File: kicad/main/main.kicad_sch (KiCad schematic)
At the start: 17 parts, among them J2 Conn_01x02, J3 Conn_01x07_Pin, J4 Conn_01x04_Pin, P1 USB_C_Plug_USB2.0, SW1 MK-12C03-G015, SW3 SW_Push, SW4 SW_Push, U1 HUSB237, U2 ZX-PH2.0-WT4P

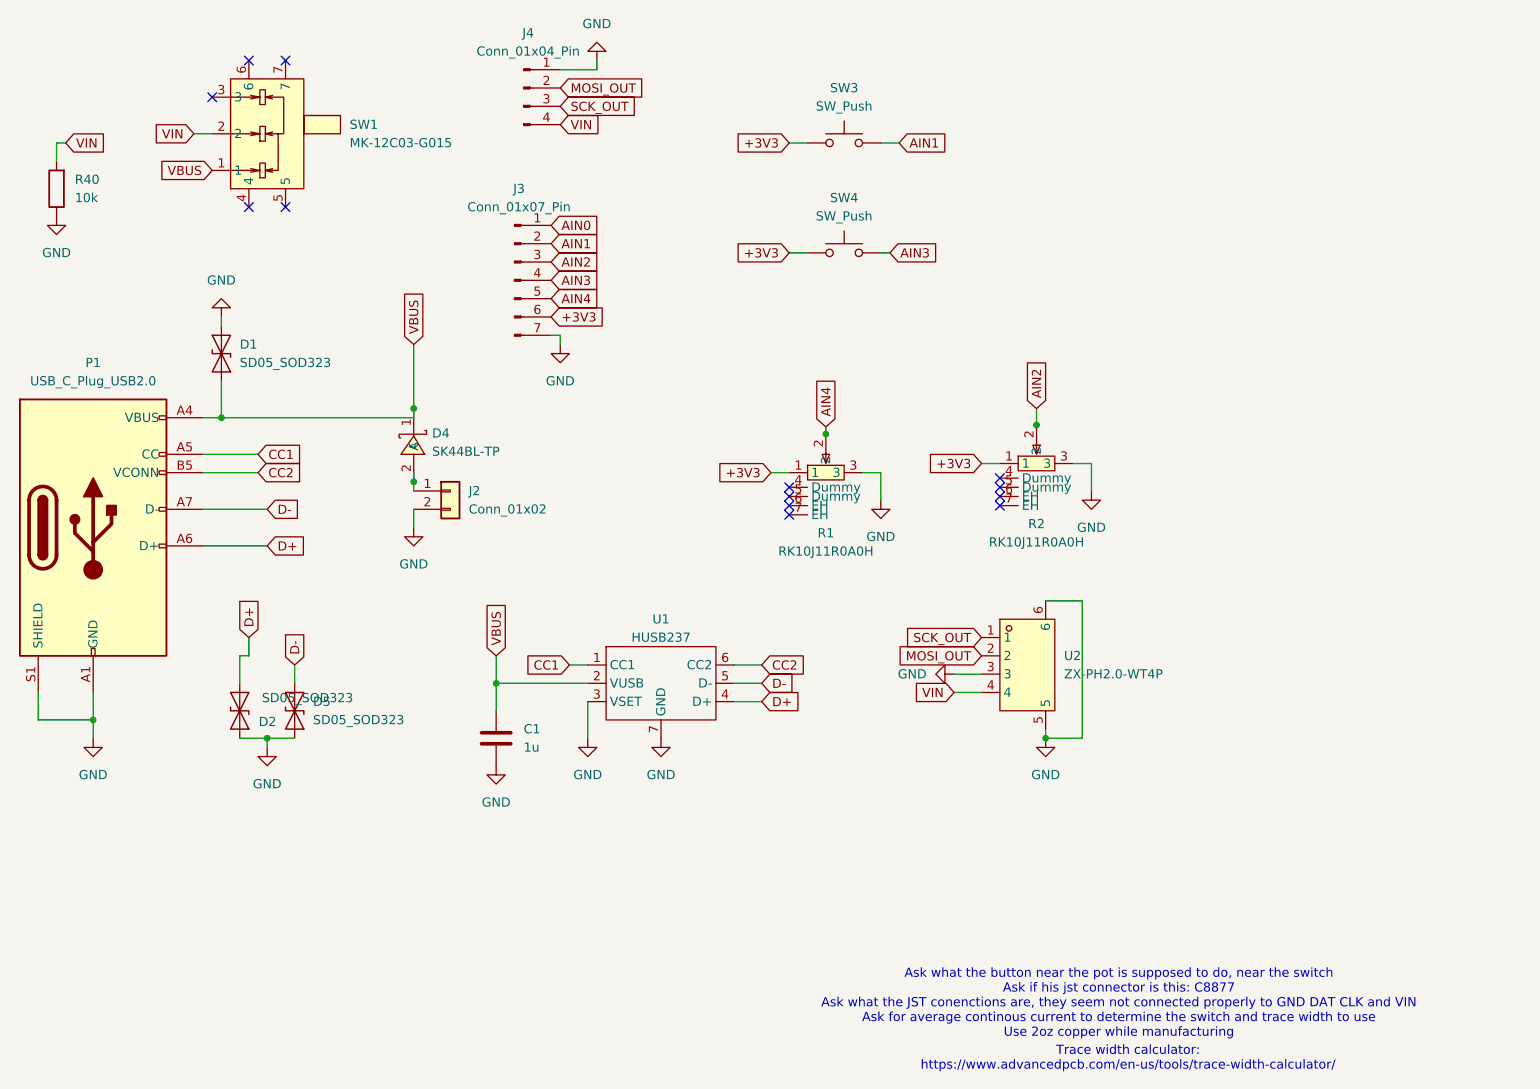
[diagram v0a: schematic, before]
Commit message: Revamped PCB
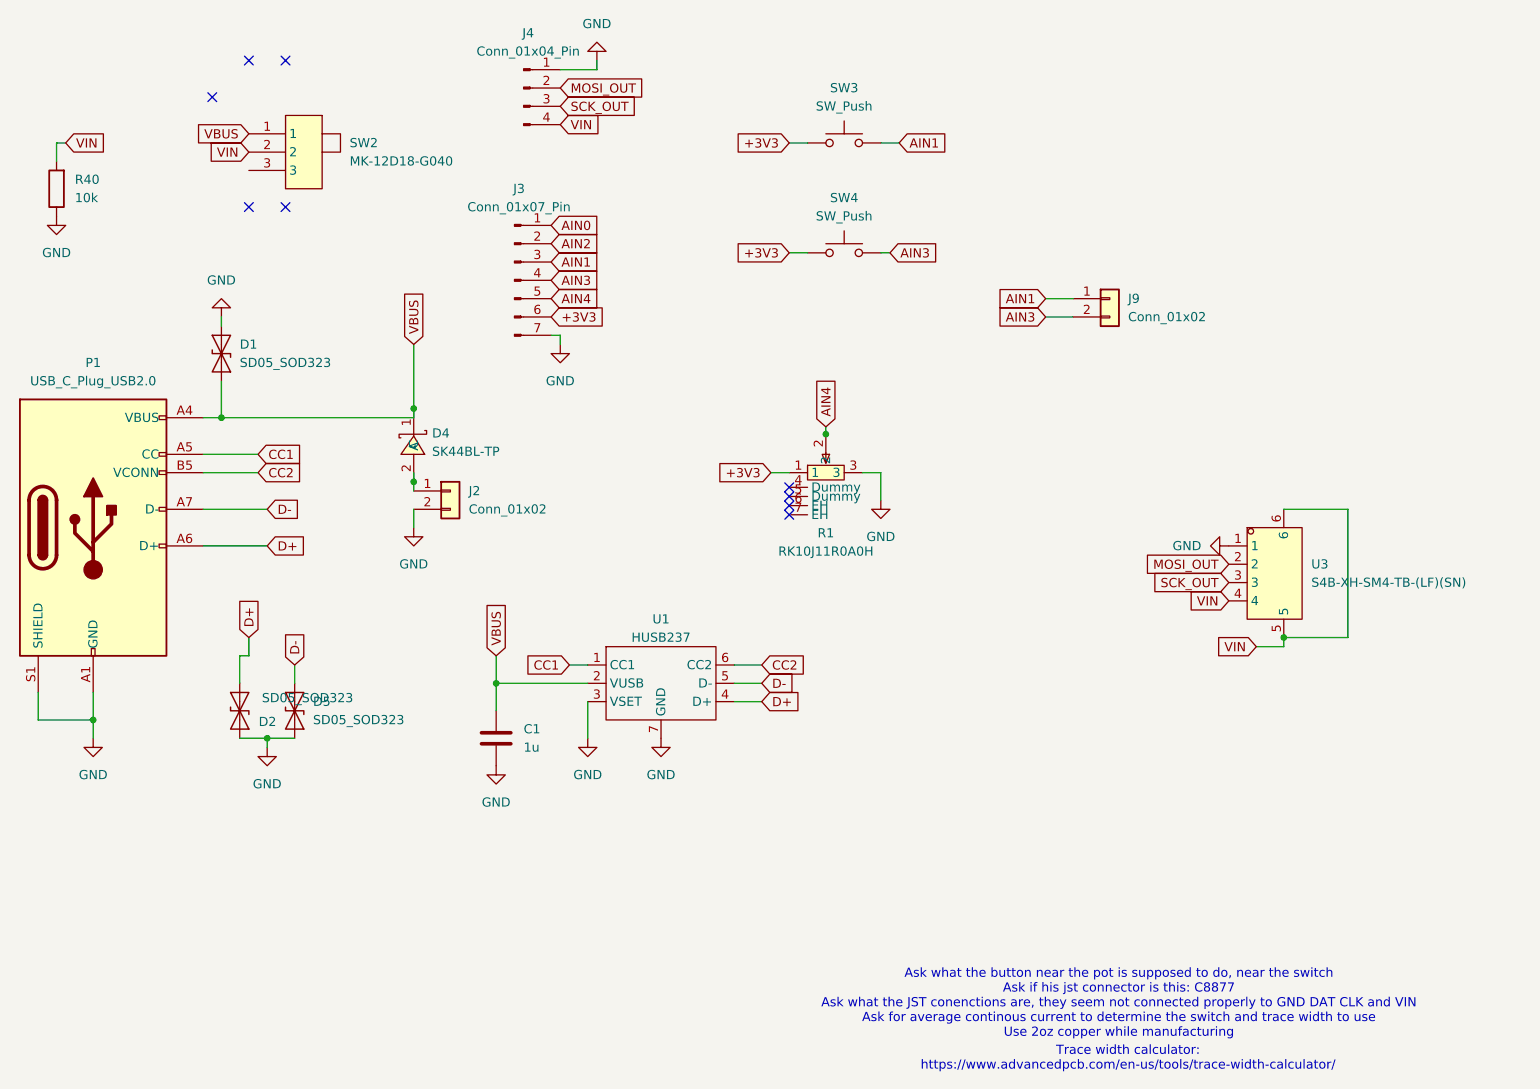
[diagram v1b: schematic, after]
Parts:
- removed R2: RK10J11R0A0H, easyeda2kicad:RES-SMD_RK10J11R0A0H, symbol easyeda2kicad:RK10J11R0A0H
- removed SW1: MK-12C03-G015, easyeda2kicad:SW-SMD_MK-12C03-G015, symbol easyeda2kicad:MK-12C03-G015
- removed U2: ZX-PH2.0-WT4P, easyeda2kicad:CONN-SMD_4P-P2.00_C2001RS10411M0101RC, symbol easyeda2kicad:ZX-PH2.0-WT4P
- added J9: Conn_01x02, symbol Connector_Generic:Conn_01x02
- added SW2: MK-12D18-G040, easyeda2kicad:SW-TH_MK-12D18-G040, symbol easyeda2kicad:MK-12D18-G040
- added U3: S4B-XH-SM4-TB-(LF)(SN), easyeda2kicad:CONN-SMD_S4B-XH-SM4-TB-LF-SN, symbol easyeda2kicad:S4B-XH-SM4-TB-(LF)(SN)
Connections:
- net AIN1: now also J3.3 (Pin_3), J9.1 (Pin_1); no longer J3.2 (Pin_2)
- net AIN2: now also J3.2 (Pin_2); no longer J3.3 (Pin_3)
- net AIN3: now also J9.2 (Pin_2)
- net GND: now also U3.1
- net MOSI_OUT: now also U3.2
- net SCK_OUT: now also U3.3
- net VBUS: now also SW2.1
- net VIN: now also SW2.2, U3.4, U3.5, U3.6
- no-connect marks 13 -> 9
